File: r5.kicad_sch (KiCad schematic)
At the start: 81 parts, among them J1 Conn_01x04, J2 Conn_01x02, SW1 SW_SPDT, SW2 SW_SPDT, SW3 SW_SPDT, SW4 SW_SPDT, U1 LMZ22005, U100 Pico, U2 74HC365, U20 DRV8871DDA, U3 GY-BNO08X, U30 DRV8871DDA, U4 PI22, U40 DRV8871DDA, U5 SDD1309, U50 DRV8871DDA, U6 3X3HEADER, U60 DRV8871DDA, U7 74HC540, U70 DRV8871DDA, U80 PCA9685PW, X1 Conn_01x02, X2 Conn_01x02, X20 Conn_01x06, X30 Conn_01x06, X40 Conn_01x06, X50 Conn_01x06, X60 Conn_01x06, X70 Conn_01x06, X81 4X3HEADER

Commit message: positions
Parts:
- removed R17: 100k, Resistor_SMD:R_0805_2012Metric, symbol Device:R
- D41: renamed from D91; JLCPCB Rotation Offset 0 -> (none)
- R16: renamed from R3; JLCPCB Rotation Offset 0 -> (none)
- R40: renamed from R14; JLCPCB Rotation Offset 0 -> (none)
- R60: renamed from R15; JLCPCB Rotation Offset 0 -> (none)
- R70: renamed from R10; JLCPCB Rotation Offset 0 -> (none)
- R80: renamed from R16; JLCPCB Rotation Offset 0 -> (none)
- U60: renamed from U80; JLCPCB Rotation Offset 0 -> (none)
- U70: renamed from U2; JLCPCB Rotation Offset (none) -> -90
- U71: renamed from U7; JLCPCB Rotation Offset (none) -> -90
- renumbered C2 to C10, C3 to C11, C30 to C21, C40 to C22, C21 to C23, C31 to C24, C41 to C25, C50 to C26, C60 to C27, C70 to C28, C51 to C29, C61 to C30, C71 to C31, C90 to C40, C80 to C60, C4 to C70, C10 to C71, C81 to C90, D90 to D40, H1 to H201, H2 to H202, H3 to H203, H4 to H204, R11 to R10, R12 to R11, R13 to R12, R1 to R13, R2 to R14, R18 to R15, R4 to R17, R30 to R21, R40 to R22, R50 to R23, R60 to R24, R70 to R25, R5 to R61, R6 to R62, R7 to R90, R8 to R91, R9 to R92, R90 to R93, R91 to R94, SW1 to SW10, SW4 to SW60, SW2 to SW70, SW3 to SW80, U1 to U10, U30 to U21, U40 to U22, U50 to U23, U60 to U24, U70 to U25, U4 to U50, U100 to U80, X1 to X10, X2 to X11, J2 to X12, X30 to X21, X40 to X22, X50 to X23, X60 to X24, X70 to X25, J1 to X40, U6 to X90, X81 to X91, U5 to X92, U3 to X93
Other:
- moved on the sheet: C60, R61, R62, R80, R93, R94, SW80

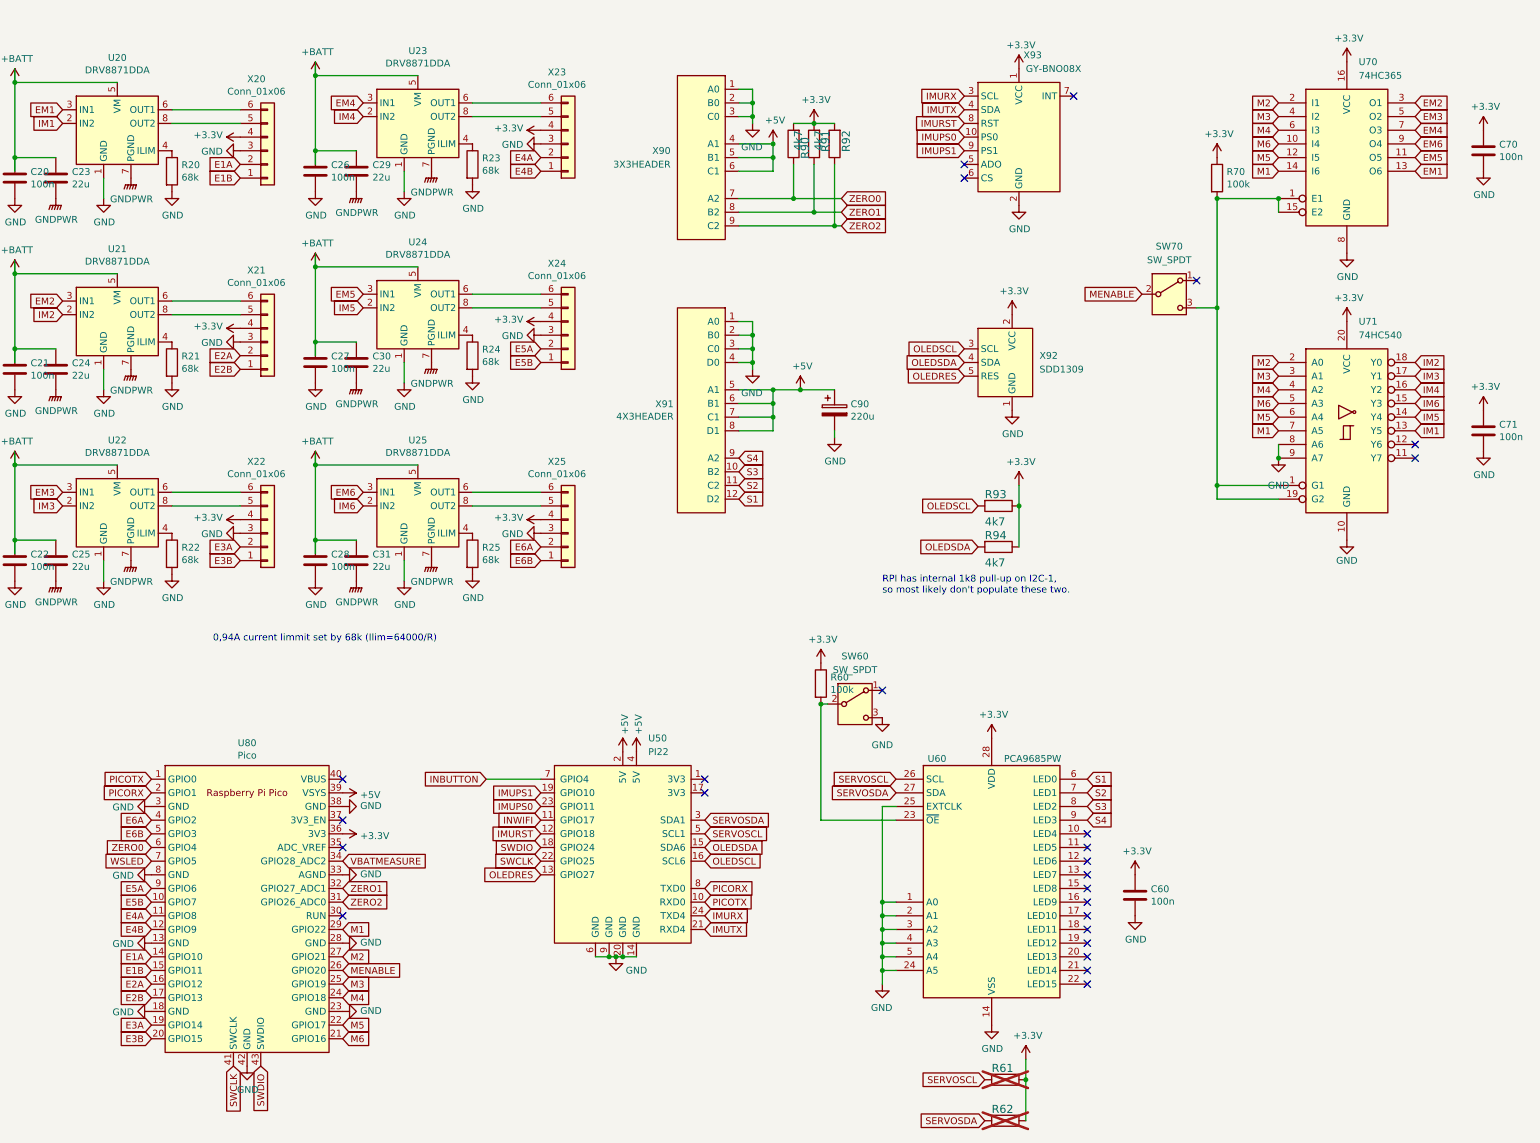
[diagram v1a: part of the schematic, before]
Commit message: start routing
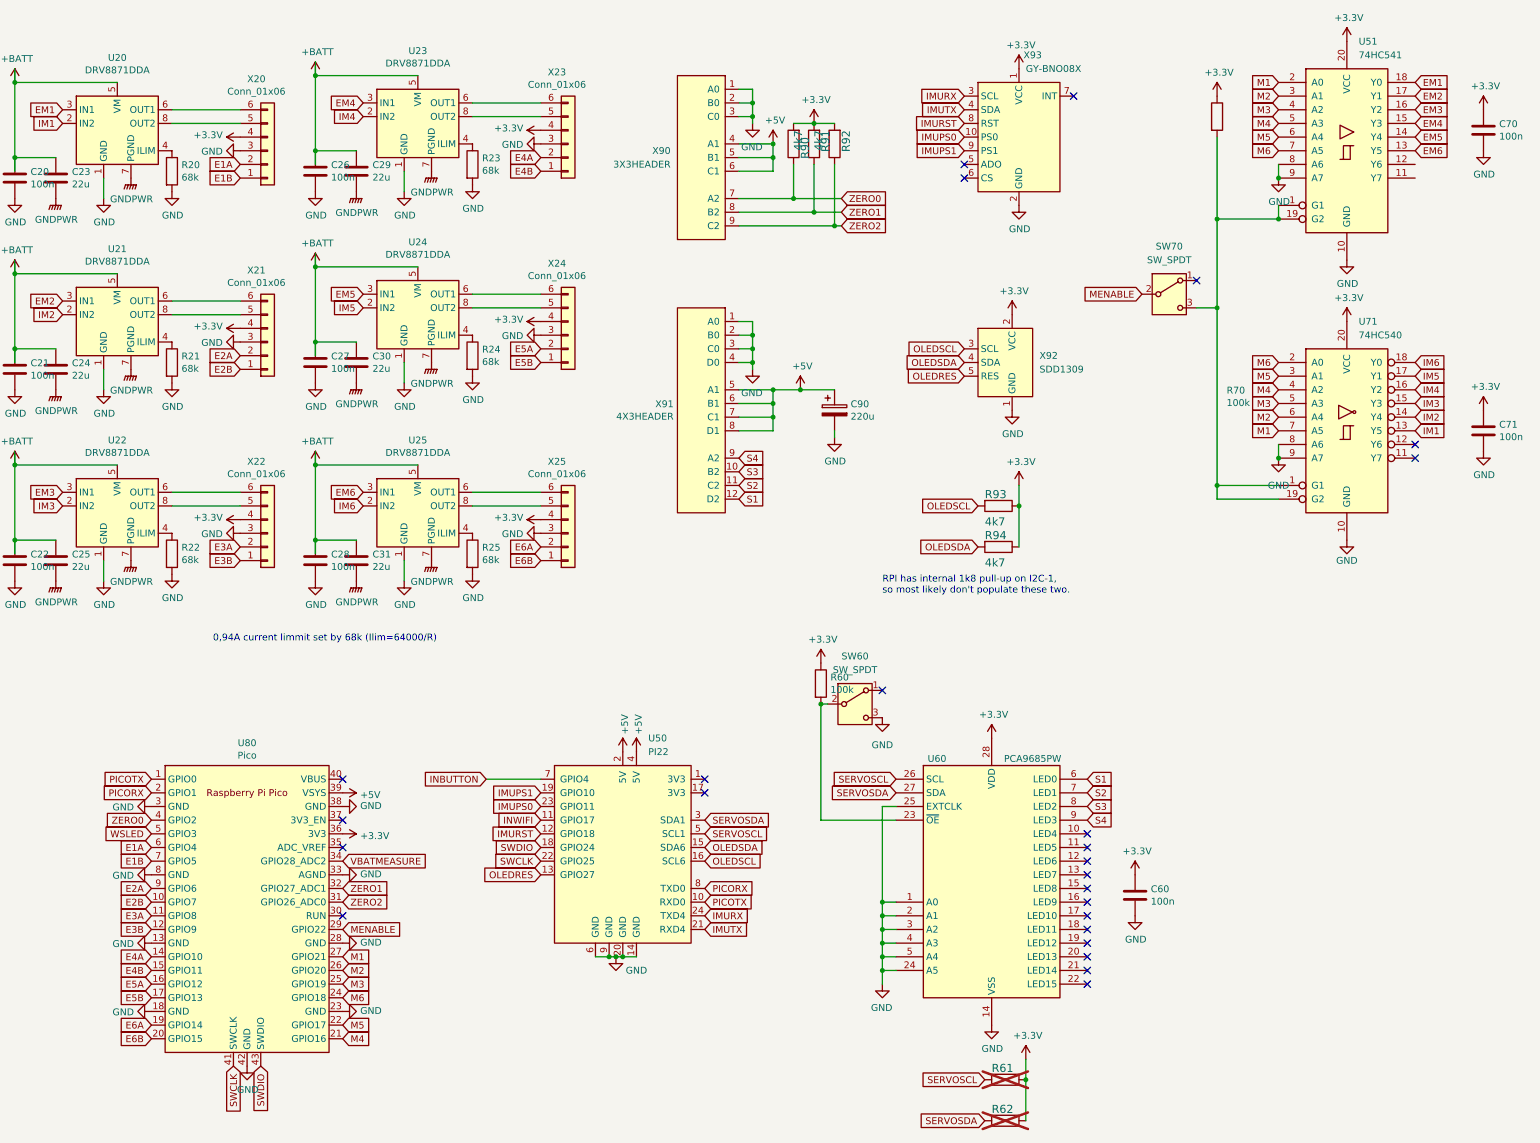
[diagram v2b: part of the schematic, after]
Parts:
- removed U70: 74HC365, Package_SO:TSSOP-16_4.4x5mm_P0.65mm, symbol 74xx:74LS365
- added U51: 74HC541, Package_SO:TSSOP-20_4.4x6.5mm_P0.65mm, symbol 74xx:74LS541
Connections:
- net +3.3V: now also U51.20 (VCC)
- net E1A: now also U80.6 (GPIO4); no longer U80.14 (GPIO10)
- net E1B: now also U80.7 (GPIO5); no longer U80.15 (GPIO11)
- net E2A: now also U80.9 (GPIO6); no longer U80.16 (GPIO12)
- net E2B: now also U80.10 (GPIO7); no longer U80.17 (GPIO13)
- net E3A: now also U80.11 (GPIO8); no longer U80.19 (GPIO14)
- net E3B: now also U80.12 (GPIO9); no longer U80.20 (GPIO15)
- net E4A: now also U80.14 (GPIO10); no longer U80.11 (GPIO8)
- net E4B: now also U80.15 (GPIO11); no longer U80.12 (GPIO9)
- net E5A: now also U80.16 (GPIO12); no longer U80.9 (GPIO6)
- net E5B: now also U80.17 (GPIO13); no longer U80.10 (GPIO7)
- net E6A: now also U80.19 (GPIO14); no longer U80.4 (GPIO2)
- net E6B: now also U80.20 (GPIO15); no longer U80.5 (GPIO3)
- net EM1: now also U51.18 (Y0)
- net EM2: now also U51.17 (Y1)
- net EM3: now also U51.16 (Y2)
- net EM4: now also U51.15 (Y3)
- net EM5: now also U51.14 (Y4)
- net EM6: now also U51.13 (Y5)
- net GND: now also U51.10 (GND), U51.8 (A6), U51.9 (A7)
- net IM2: now also U71.14 (Y4); no longer U71.18 (Y0)
- net IM3: now also U71.15 (Y3); no longer U71.17 (Y1)
- net IM5: now also U71.17 (Y1); no longer U71.14 (Y4)
- net IM6: now also U71.18 (Y0); no longer U71.15 (Y3)
- net M1: now also U80.27 (GPIO21), U51.2 (A0); no longer U80.29 (GPIO22)
- net M2: now also U71.6 (A4), U80.26 (GPIO20), U51.3 (A1); no longer U71.2 (A0), U80.27 (GPIO21)
- net M3: now also U71.5 (A3), U51.4 (A2); no longer U71.3 (A1)
- net M4: now also U80.21 (GPIO16), U51.5 (A3); no longer U80.24 (GPIO18)
- net M5: now also U71.3 (A1), U51.6 (A4); no longer U71.6 (A4)
- net M6: now also U71.2 (A0), U80.24 (GPIO18), U51.7 (A5); no longer U71.5 (A3), U80.21 (GPIO16)
- net MENABLE: now also U80.29 (GPIO22); no longer U80.26 (GPIO20)
- net WSLED: now also U80.5 (GPIO3); no longer U80.7 (GPIO5)
- net ZERO0: now also U80.4 (GPIO2); no longer U80.6 (GPIO4)
- net at R70.2, SW70.3 (C), U71.1 (G1)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: now also U51.1 (G1), U51.19 (G2)
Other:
- moved on the sheet: C70, R70
